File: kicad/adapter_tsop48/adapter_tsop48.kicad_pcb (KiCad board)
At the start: 2 copper layers, 48 x 33 mm, 3 parts, among them J1 Conn_02x12_Odd_Even_1, J2 Conn_02x12_Odd_Even_2, P1 TSOP-48_adapter

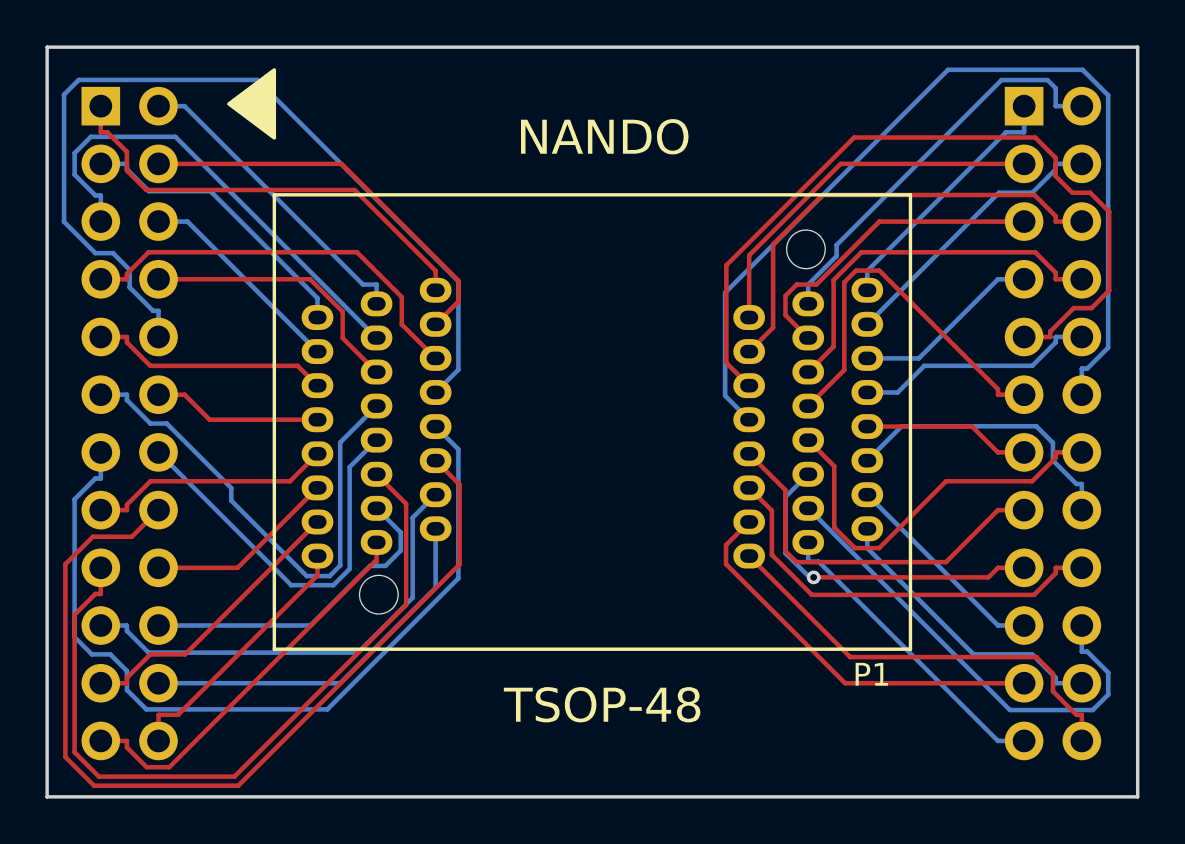
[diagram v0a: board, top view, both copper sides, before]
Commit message: update PCB design and cleanup KiCad files
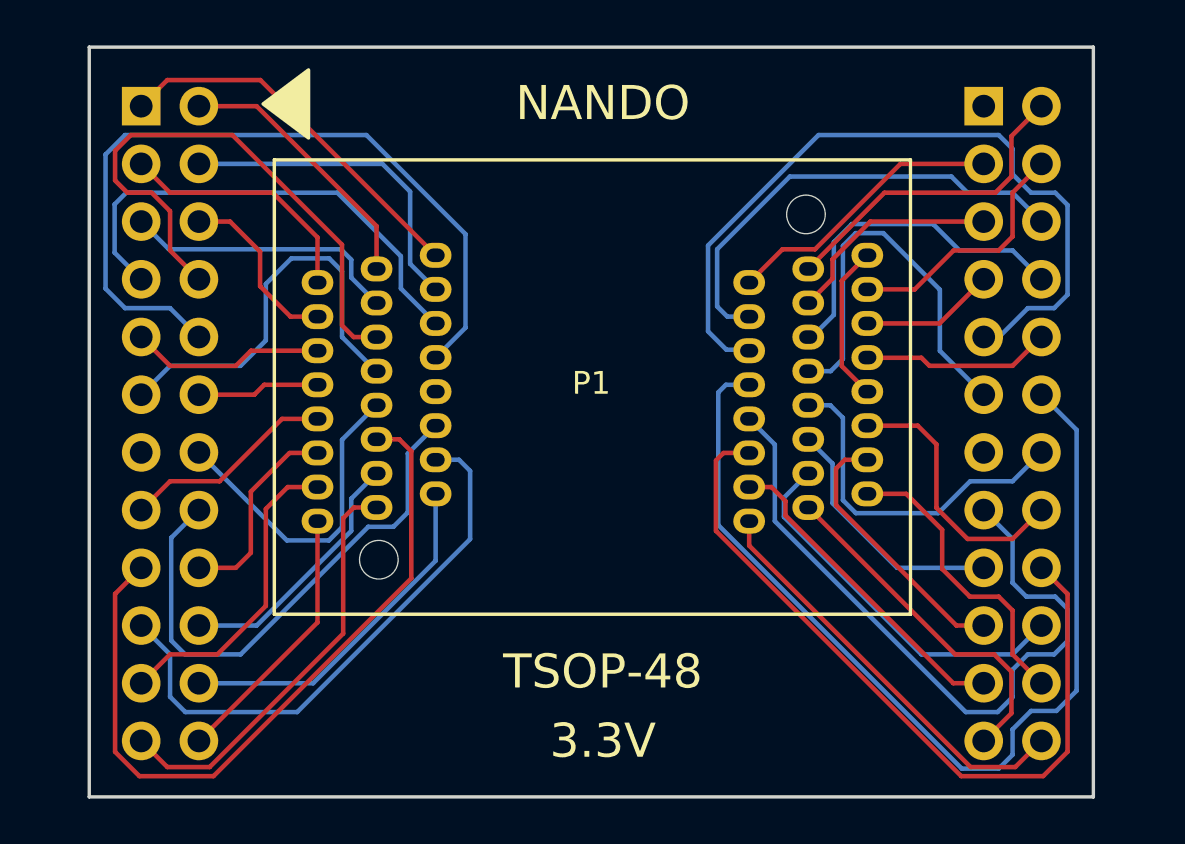
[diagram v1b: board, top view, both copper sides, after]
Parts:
- J1: footprint lib_fp:PinSocket_2x12_P2.54mm_Vertical -> Connector_PinSocket_2.54mm:PinSocket_2x12_P2.54mm_Vertical
- moved J2 1.78 mm to (141.2, 85.6)
- moved J1 1.78 mm to (104.1, 85.6)
- moved P1 1.54 mm to (138.0, 88.0)
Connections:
- J1 pad 13: Net-(J1-Pad13) -> GND
- J2 pad 25: Net-(J2-Pad25) -> GND
- J2 pad 36: Net-(J2-Pad36) -> GND
- J2 pad 48: Net-(J2-Pad48) -> GND
- P1 pad 13: Net-(J1-Pad13) -> GND
- P1 pad 25: Net-(J2-Pad25) -> GND
- P1 pad 36: Net-(J2-Pad36) -> GND
- P1 pad 48: Net-(J2-Pad48) -> GND
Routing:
- net Net-(J1-Pad13): track 36.9 -> 0.00 mm
- net GND: track 0.00 -> 25.4 mm
- net Net-(J2-Pad25): track 19.1 -> 0.00 mm
- net Net-(J1-Pin_16): track 40.5 -> 23.8 mm
- net Net-(J2-Pin_31): track 18.4 -> 33.7 mm
- net Net-(J2-Pin_34): track 16.6 -> 31.4 mm
- net Net-(J1-Pin_8): track 12.0 -> 25.4 mm
- net Net-(J2-Pad48): track 11.4 -> 0.00 mm
- net Net-(J1-Pin_5): track 20.9 -> 12.3 mm
- net Net-(J2-Pad36): track 7.37 -> 0.00 mm
- net Net-(J1-Pin_10): track 39.6 -> 34.9 mm
- net Net-(J1-Pin_19): track 20.3 -> 25.0 mm
- net Net-(J2-Pin_44): track 14.1 -> 9.71 mm
- net Net-(J1-Pin_11): track 22.2 -> 18.1 mm
- net Net-(J2-Pin_29): track 20.8 -> 16.7 mm
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- added copper zone on B.Cu, net GND
- added copper zone on F.Cu, net GND
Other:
- board size 48 x 33 mm -> 44.2 x 33 mm
- net class Default removed
- board text added: "3.3V"
